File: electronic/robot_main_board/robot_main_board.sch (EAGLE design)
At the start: 28 parts, among them J1 HORIZONTAL_ROTATE, J10 joint2_ends_min, J11 joint2_ends_max, J13 hr_ends_max, J2 JOINT_1, J3 JOINT_2, J4 JOYSTICK, J5 joint1_en_sw, J6 joint2_en_sw, J7 hr_en_sw, J8 joint1_ends_min, J9 joint1_ends_max

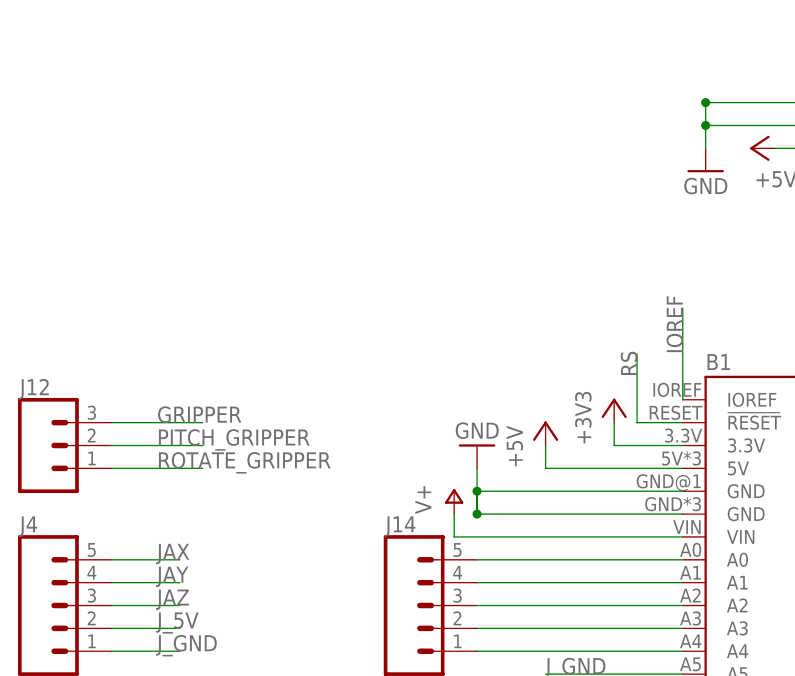
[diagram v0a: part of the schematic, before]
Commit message: change robot_main_board
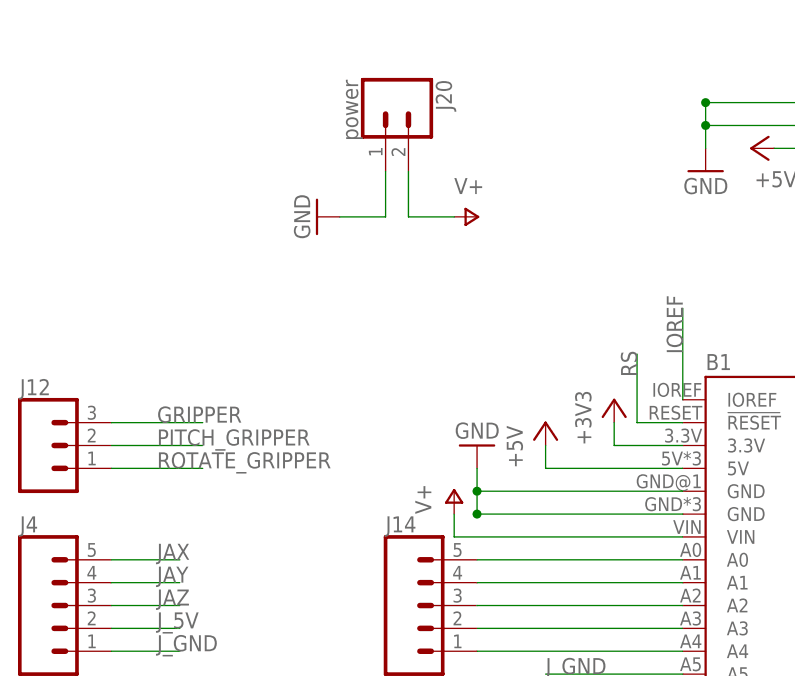
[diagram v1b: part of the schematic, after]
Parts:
- added J20: power, SparkFun-Connectors:CONN_02POLAR
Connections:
- net GND: now also J20.1
- net V+: now also J20.2
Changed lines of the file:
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@@
 <part name="J18" library="SparkFun-Connectors" deviceset="CONN_07" device=""/>
 <part name="J19" library="SparkFun-Connectors" deviceset="CONN_05" device=""/>
+<part name="J20" library="SparkFun-Connectors" deviceset="CONN_02" device="POLAR" value="power"/>
+<part name="GND12" library="supply1" library_urn="urn:adsk.eagle:library:371" deviceset="GND" device=""/>
+<part name="P+13" library="supply1" library_urn="urn:adsk.eagle:library:371" deviceset="V+" device=""/>
 </parts>
 <sheets>
@@
 <instance part="J18" gate="G$1" x="127" y="180.34" rot="R180"/>
 <instance part="J19" gate="G$1" x="149.86" y="48.26" rot="R180"/>
+<instance part="J20" gate="G$1" x="50.8" y="182.88" rot="R270"/>
+<instance part="GND12" gate="1" x="43.18" y="170.18" rot="R270"/>
+<instance part="P+13" gate="1" x="60.96" y="170.18" rot="R270"/>
 </instances>
 <busses>
@@
 <wire x1="60.96" y1="142.24" x2="60.96" y2="139.7" width="0.1524" layer="91"/>
 <pinref part="B1" gate="B1" pin="GND"/>
-<wire x1="60.96" y1="139.7" x2="60.96" y2="137.16" width="0.1524" layer="91"/>
 <wire x1="60.96" y1="137.16" x2="83.82" y2="137.16" width="0.1524" layer="91"/>
 <pinref part="B1" gate="B1" pin="GND@2"/>
@@
 <pinref part="J18" gate="G$1" pin="3"/>
 </segment>
+<segment>
+<pinref part="GND12" gate="1" pin="GND"/>
+<pinref part="J20" gate="G$1" pin="1"/>
+<wire x1="45.72" y1="170.18" x2="50.8" y2="170.18" width="0.1524" layer="91"/>
+<wire x1="50.8" y1="170.18" x2="50.8" y2="175.26" width="0.1524" layer="91"/>
+</segment>
 </net>
 <net name="+5V" class="0">
@@
 <wire x1="58.42" y1="134.62" x2="83.82" y2="134.62" width="0.1524" layer="91"/>
 </segment>
-</net>
+<segment>
+<pinref part="J20" gate="G$1" pin="2"/>
+<wire x1="53.34" y1="175.26" x2="53.34" y2="170.18" width="0.1524" layer="91"/>
+<pinref part="P+13" gate="1" pin="V+"/>
+<wire x1="53.34" y1="170.18" x2="58.42" y2="170.18" width="0.1524" layer="91"/>
+</segment>
+</net>
